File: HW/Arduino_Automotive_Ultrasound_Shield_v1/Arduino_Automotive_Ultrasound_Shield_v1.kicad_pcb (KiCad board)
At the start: 2 copper layers, 9 parts, among them J1 Conn_01x04_Socket, J2 Conn_01x04_Socket, J3 Barrel_Jack_Switch, J4 Conn_01x04_Socket, J5 1x3 2.54mm male, J6 1x3 2.54mm male, SW1 SW_Push, U2 LM7805_TO220

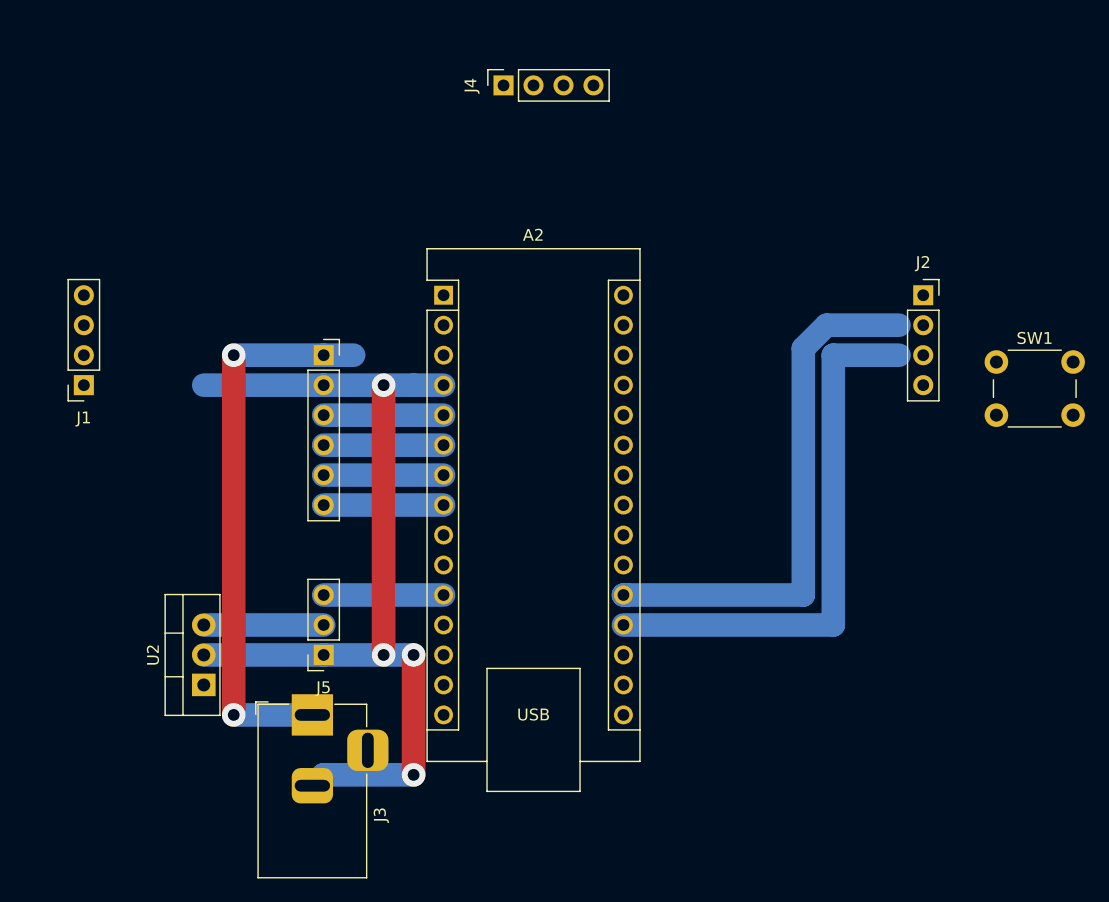
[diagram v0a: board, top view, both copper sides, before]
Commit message: pcb
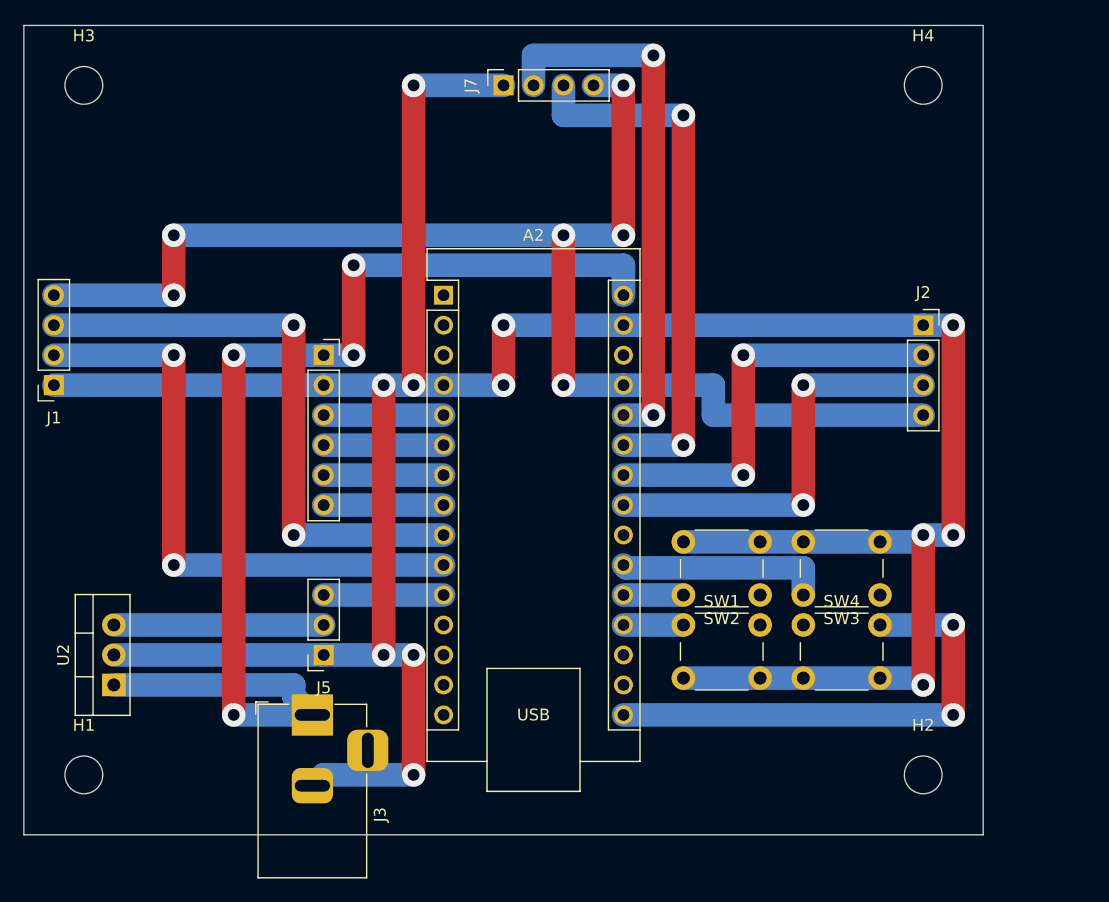
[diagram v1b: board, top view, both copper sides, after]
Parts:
- removed J4: Conn_01x04_Socket, Connector_PinSocket_2.54mm:PinSocket_1x04_P2.54mm_Vertical
- added H1: M3, MountingHole:MountingHole_3.2mm_M3, F.Cu at (86.4, 91.4)
- added H2: M3, MountingHole:MountingHole_3.2mm_M3, F.Cu at (157.5, 91.4)
- added H3: M3, MountingHole:MountingHole_3.2mm_M3, F.Cu at (86.4, 33.0)
- added H4: M3, MountingHole:MountingHole_3.2mm_M3, F.Cu at (157.5, 33.0)
- added J7: 1x4 2.54mm female, Connector_PinSocket_2.54mm:PinSocket_1x04_P2.54mm_Vertical, F.Cu at (121.9, 33.0)
- added SW2: SW_Push, Button_Switch_THT:SW_PUSH_6mm, F.Cu at (143.7, 76.2)
- added SW3: SW_Push, Button_Switch_THT:SW_PUSH_6mm, F.Cu at (153.8, 76.2)
- added SW4: SW_Push, Button_Switch_THT:SW_PUSH_6mm, F.Cu at (147.3, 78.7)
- J1, J2: value Conn_01x04_Socket -> 1x4 2.54mm female
- moved SW1 34.6 mm to (137.2, 78.7)
- moved U2 7.62 mm to (88.9, 83.8)
- moved J1 2.54 mm to (83.8, 58.4)
- moved J2 2.54 mm to (157.5, 53.3)
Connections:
- A2 pad 10: Net-(A2-D7) -> /ECHO_2
- A2 pad 16: unconnected-(A2-SCK-Pad16) -> /PB3
- A2 pad 19: /ECHO_0 -> /PB0
- A2 pad 20: /TRIG_0 -> /PB1
- A2 pad 21: unconnected-(A2-A2-Pad21) -> /PB2
- A2 pad 23: unconnected-(A2-SDA/A4-Pad23) -> /TRIG_1
- A2 pad 24: unconnected-(A2-SCL/A5-Pad24) -> /ECHO_1
- A2 pad 25: unconnected-(A2-A6-Pad25) -> /TRIG_0
- A2 pad 26: unconnected-(A2-A7-Pad26) -> /ECHO_0
- A2 pad 9: Net-(A2-D6) -> /TRIG_2
- J1 pad 1: (no net) -> GND
- J1 pad 2: (no net) -> /ECHO_2
- J1 pad 3: (no net) -> /TRIG_2
- J1 pad 4: (no net) -> +5V
- J2 pad 1: (no net) -> GND
- J2 pad 2: (no net) -> /ECHO_1
- J2 pad 3: (no net) -> /TRIG_1
- J2 pad 4: (no net) -> +5V
- SW1 pad 1: unconnected-(SW1-Pad1) -> /PB0
- SW1 pad 2: unconnected-(SW1-Pad2) -> GND
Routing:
- net GND: track 80.1 -> 255.8 mm, vias 4 -> 12
- net +5V: track 0.00 -> 114.3 mm, vias 0 -> 6
- net +12V: track 47.3 -> 98.8 mm, vias 2 -> 4
- net /TRIG_2: track 0.00 -> 50.8 mm, vias 0 -> 2
- net /ECHO_2: track 0.00 -> 50.8 mm, vias 0 -> 2
- net /PB3: track 0.00 -> 41.8 mm, vias 0 -> 2
- net /ECHO_1: track 0.00 -> 35.6 mm, vias 0 -> 2
- net /TRIG_1: track 0.00 -> 35.6 mm, vias 0 -> 2
- net /PB2: track 0.00 -> 17.6 mm
- net Vdrive: track 10.2 -> 17.8 mm
- net /PB1: track 0.00 -> 5.08 mm
- net /PB0: track 0.00 -> 5.08 mm
- net /ECHO_0: track 46.2 -> 45.7 mm, vias 0 -> 2
- net /TRIG_0: track 45.3 -> 45.7 mm, vias 0 -> 2
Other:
- board outline added: 81.3 x 68.6 mm
